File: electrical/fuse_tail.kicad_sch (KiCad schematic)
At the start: 3 parts, among them U10 TAIL LIGHT, U13 BEACON, U9 PITCH TRIM

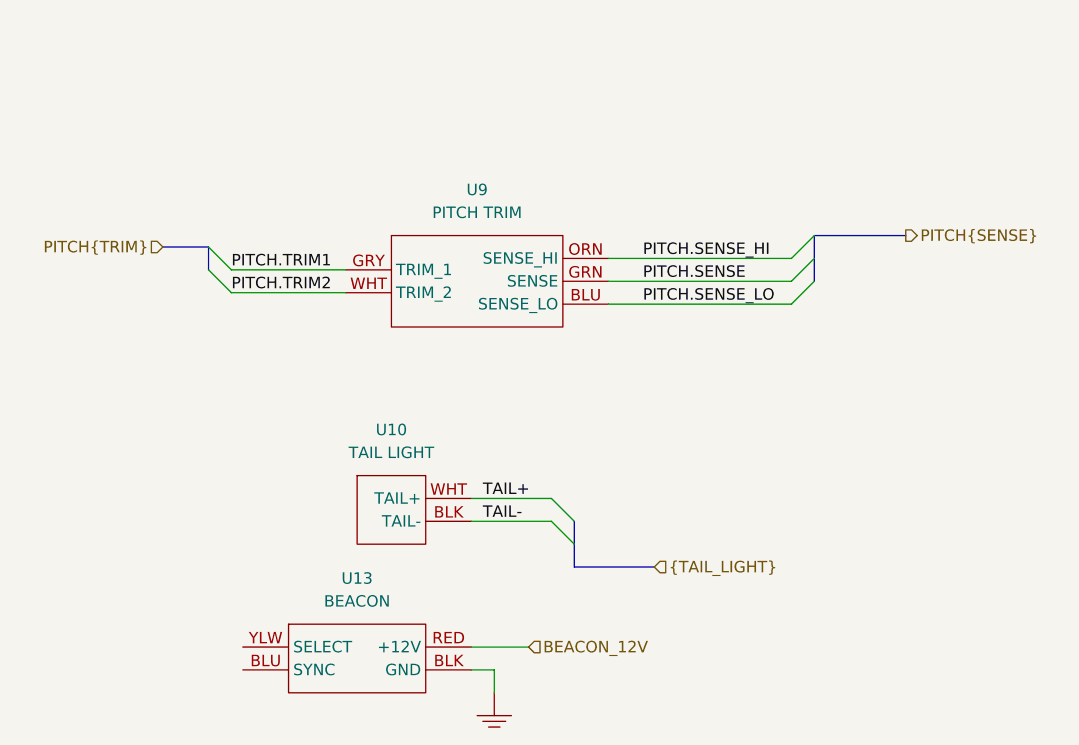
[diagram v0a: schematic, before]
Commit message: 🎮 Working on electrical schematic
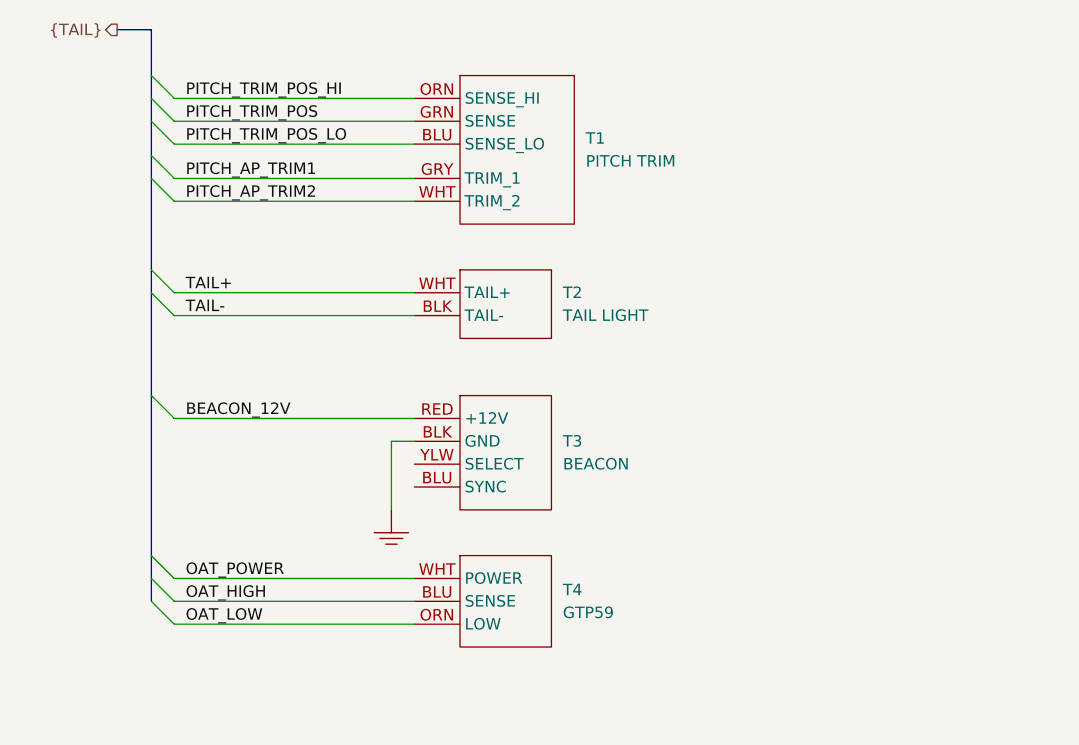
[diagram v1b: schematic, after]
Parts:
- added T4: GTP59, symbol Garmin:GTP59
- renumbered U9 to T1, U10 to T2, U13 to T3
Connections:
- net PITCH.SENSE renamed PITCH_TRIM_POS
- net PITCH.SENSE_HI renamed PITCH_TRIM_POS_HI
- net PITCH.SENSE_LO renamed PITCH_TRIM_POS_LO
- net PITCH.TRIM1 renamed PITCH_AP_TRIM1
- net PITCH.TRIM2 renamed PITCH_AP_TRIM2
- new net OAT_HIGH: T4.BLU (SENSE)
- new net OAT_LOW: T4.ORN (LOW)
- new net OAT_POWER: T4.WHT (POWER)
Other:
- moved on the sheet: T1, T2, T3
